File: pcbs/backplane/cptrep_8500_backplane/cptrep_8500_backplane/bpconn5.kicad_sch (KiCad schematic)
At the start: 1 part, among them J5 cpt-backplane_100

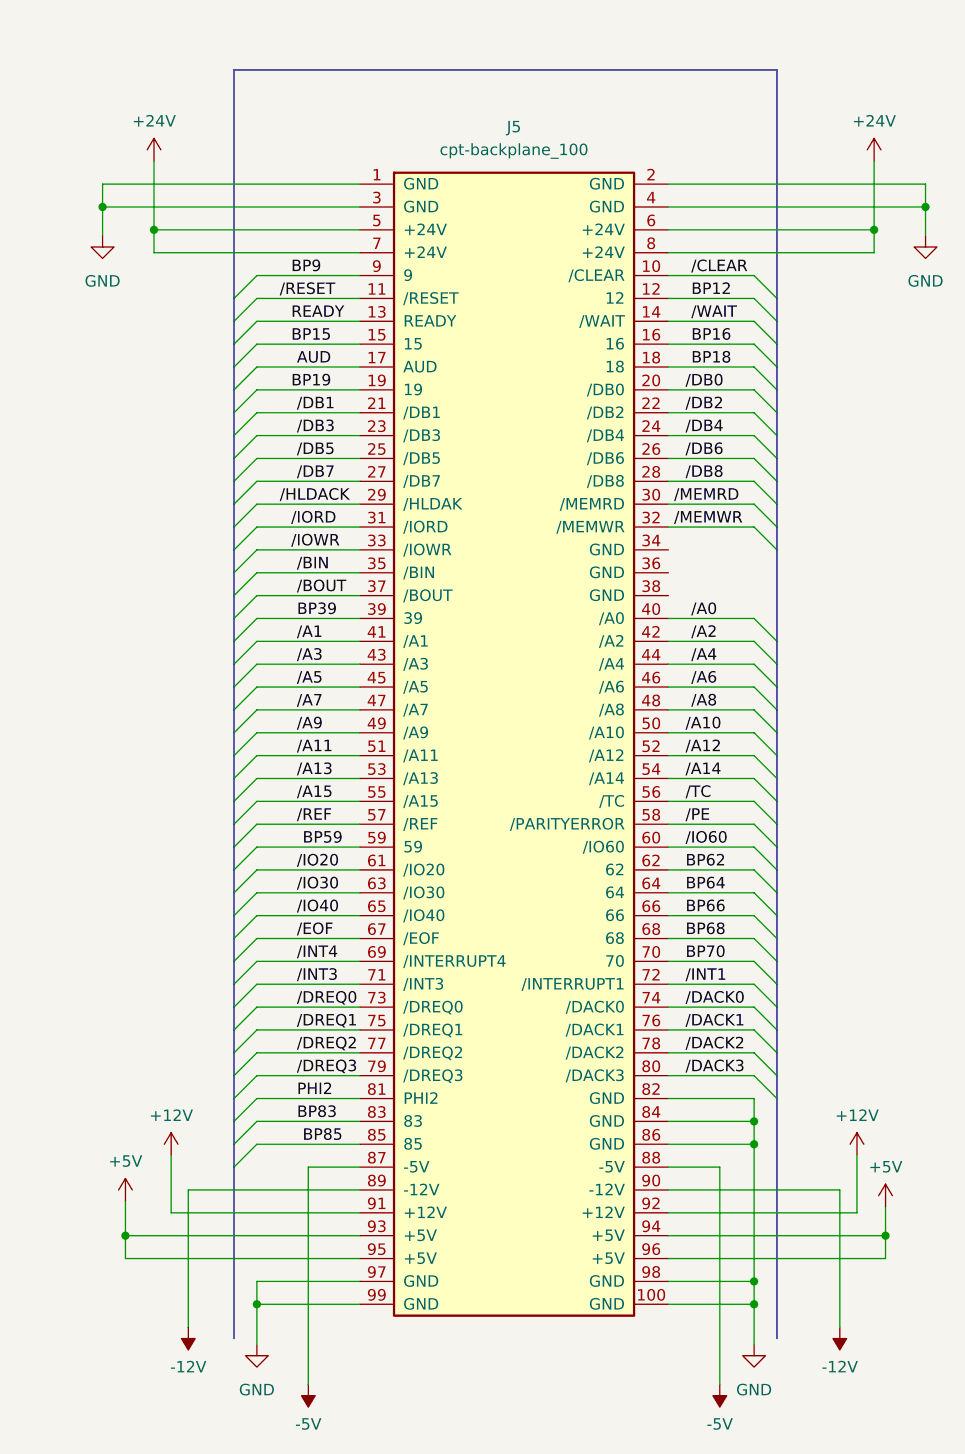
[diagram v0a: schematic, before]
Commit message: "Update"
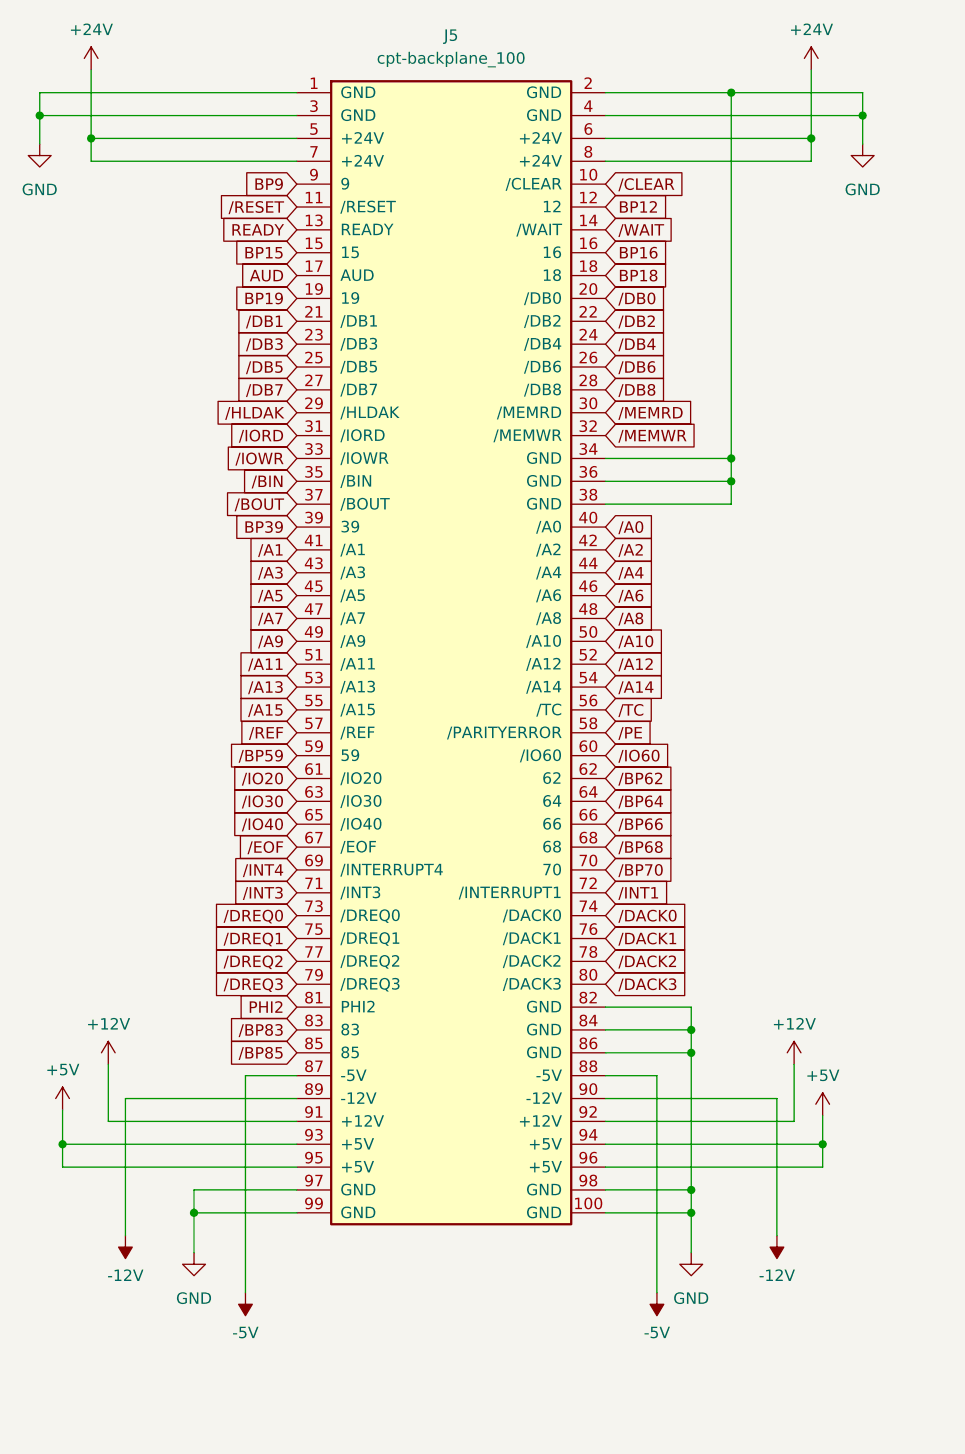
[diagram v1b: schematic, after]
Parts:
- J5: footprint (none) -> ajm-cpt:cpt-8500-backplane-connector
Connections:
- net GND: now also J5.34 (GND), J5.36 (GND), J5.38 (GND)
- net /BP68: now reaches J5.68
- net BP59 renamed /BP59
- net BP62 renamed /BP62
- net BP64 renamed /BP64
- net BP66 renamed /BP66
- net BP70 renamed /BP70
- net BP83 renamed /BP83
- net BP85 renamed /BP85
- net /HLDACK renamed /HLDAK
